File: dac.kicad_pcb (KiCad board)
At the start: 2 copper layers, 20 parts, among them J1 RCJ-2121, J2 Conn_01x03_Male, SW1 SW_DIP_x01, U1 pcm5102a

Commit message: correcciones profe
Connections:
- C11 pad 1: GNDA -> +3.3VA
- C11 pad 2: +3.3VA -> GNDA

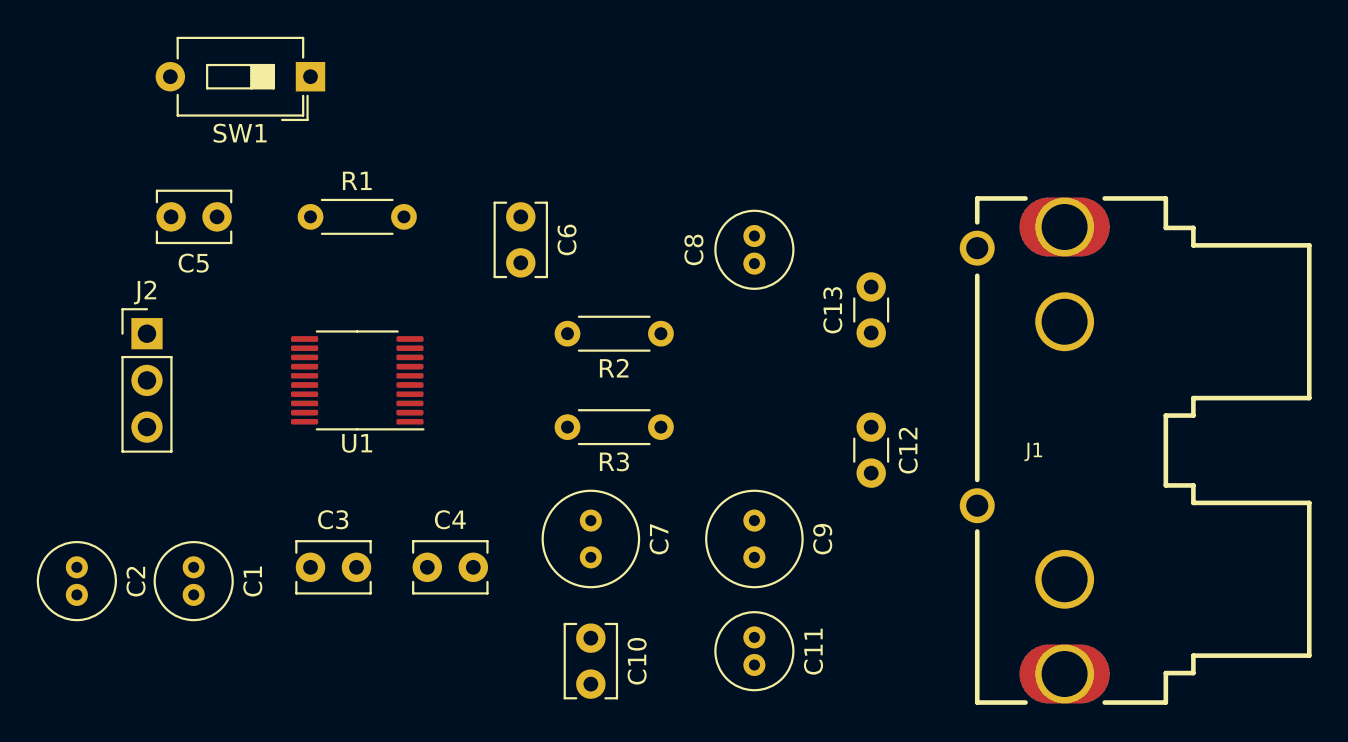
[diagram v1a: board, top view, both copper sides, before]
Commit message: ruteo PCB
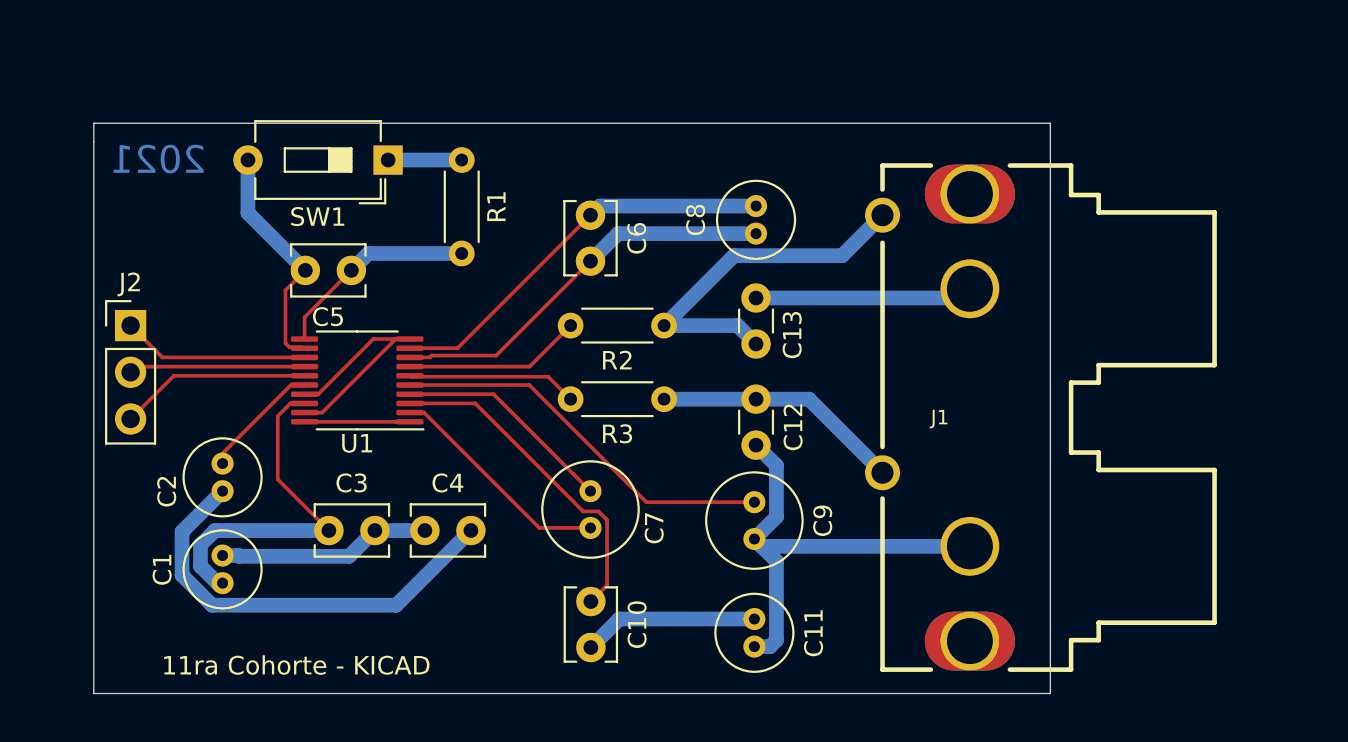
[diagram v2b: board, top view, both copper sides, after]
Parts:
- moved C2 8.94 mm to (140.0, 100.0), turned to 90 degrees
- moved R1 8.78 mm to (153.0, 82.0), turned to 270 degrees
- moved C5 7.86 mm to (147.0, 88.0)
- moved C12 6.44 mm to (169.0, 95.0)
- moved C13 6.29 mm to (169.0, 92.0)
- moved SW1 6.19 mm to (149.0, 82.0)
- moved J1 5.45 mm to (179.0, 96.0)
- moved C6 3.79 mm to (160.0, 85.0)
- moved C3 2.24 mm to (145.8, 102.1)
- moved C4 2.00 mm to (151.0, 102.1)
- moved C10 1.99 mm to (160.0, 106.0)
- moved C1 1.79 mm to (140.0, 105.0), turned to 90 degrees
- moved C8 1.63 mm to (169.0, 86.0)
- moved C7 1.60 mm to (160.0, 100.0)
- moved R3 1.53 mm to (164.0, 95.0)
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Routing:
- net GNDA: track 0.00 -> 78.0 mm
- net +3.3VA: track 0.00 -> 61.2 mm
- net Earth: track 0.00 -> 46.1 mm
- net Net-(C9-Pad1): track 0.00 -> 21.4 mm
- net Net-(C13-Pad1): track 0.00 -> 19.8 mm
- net Net-(C1-Pad1): track 0.00 -> 19.2 mm
- net Net-(C12-Pad1): track 0.00 -> 13.5 mm
- net Net-(C7-Pad2): track 0.00 -> 12.4 mm
- net Net-(C7-Pad1): track 0.00 -> 12.0 mm
- net Net-(C5-Pad1): track 0.00 -> 11.2 mm
- net Net-(J2-Pad3): track 0.00 -> 10.4 mm
- net Net-(J2-Pad1): track 0.00 -> 10.2 mm
- net Net-(R2-Pad2): track 0.00 -> 9.66 mm
- net Net-(J2-Pad2): track 0.00 -> 9.59 mm
- net Net-(R3-Pad2): track 0.00 -> 9.26 mm
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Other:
- board outline added: 52 x 31 mm
- board text added: "11ra Cohorte - KICAD"
- board text added: "2021"
